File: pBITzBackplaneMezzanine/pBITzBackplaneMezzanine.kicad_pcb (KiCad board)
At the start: 4 copper layers, 99.9 x 80.4 mm, 41 parts, among them J1 USB3_A_Stacked, J2 Conn_01x04, J3 Conn_01x04, J4 10067847-001RLF, J5 Conn_02x10_Odd_Even, U1 FE1.1S-BSOP28BCN, U2 MAX3421EETJ_T, U3 CD74HC4050M96, U4 CD74HC4050M96, Y1 ABL-12.000MHZ-B2, Y2 ABL-12.000MHZ-B2

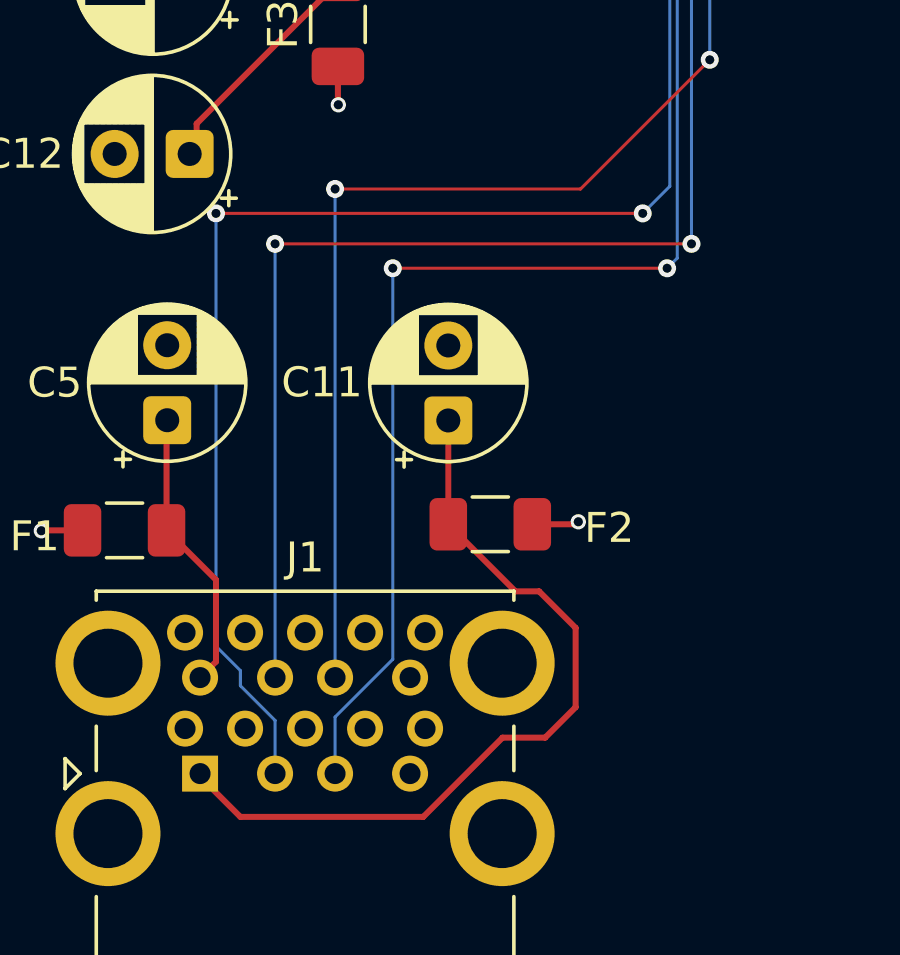
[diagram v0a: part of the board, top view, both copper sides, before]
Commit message: First pass of validation
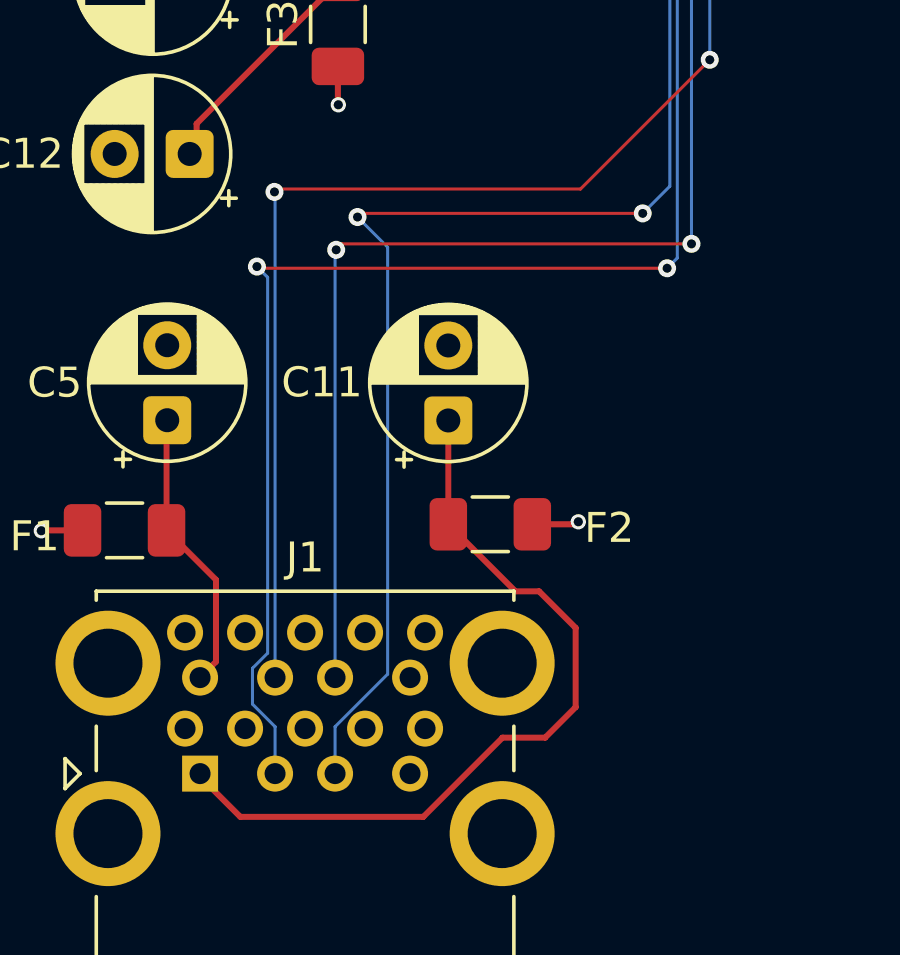
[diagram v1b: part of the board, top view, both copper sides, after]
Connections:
- J1 pad 11: /USBPorts/DP2 -> /USBPorts/DM2
- J1 pad 12: /USBPorts/DM2 -> /USBPorts/DP2
- J1 pad 2: /USBPorts/DP1 -> /USBPorts/DM1
- J1 pad 3: /USBPorts/DM1 -> /USBPorts/DP1
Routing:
- net /USBPorts/DM1: track 59.1 -> 63.6 mm
- net /USBPorts/DP1: track 63.3 -> 58.8 mm
- net /USBPorts/DP2: track 61.0 -> 58.9 mm
- net /USBPorts/DM2: track 58.7 -> 60.7 mm
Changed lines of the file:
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@@
 			(layers "*.Cu" "*.Mask")
 			(remove_unused_layers no)
-			(net "/USBPorts/DP1")
+			(net "/USBPorts/DM1")
 			(pinfunction "D1-_2")
 			(pintype "bidirectional")
@@
 			(layers "*.Cu" "*.Mask")
 			(remove_unused_layers no)
-			(net "/USBPorts/DM1")
+			(net "/USBPorts/DP1")
 			(pinfunction "D1+_3")
 			(pintype "bidirectional")
@@
 			(layers "*.Cu" "*.Mask")
 			(remove_unused_layers no)
-			(net "/USBPorts/DP2")
+			(net "/USBPorts/DM2")
 			(pinfunction "D2-_11")
 			(pintype "bidirectional")
@@
 			(layers "*.Cu" "*.Mask")
 			(remove_unused_layers no)
-			(net "/USBPorts/DM2")
+			(net "/USBPorts/DP2")
 			(pinfunction "D2+_12")
 			(pintype "bidirectional")
@@
 			)
 		)
-		(property "KiLib_Generator" "mounting_hardware/mounting_hole"
-			(at 0 0 0)
-			(layer "F.SilkS")
-			(hide yes)
-			(effects
-				(font
-					(size 1 1)
-					(thickness 0.15)
-				)
-			)
-		)
 		(property ki_fp_filters "MountingHole*Pad*")
 		(sheetname "/MezzanineConnector/")
@@
 			)
 		)
-		(property "KiLib_Generator" "connector/pin_header_socket"
-			(at 0 0 90)
-			(layer "F.SilkS")
-			(hide yes)
-			(effects
-				(font
-					(size 1 1)
-					(thickness 0.15)
-				)
-			)
-		)
 		(property "Field5" ""
 			(at 0 0 90)
@@
 			)
 		)
-		(property "KiLib_Generator" "mounting_hardware/mounting_hole"
-			(at 0 0 0)
-			(layer "F.SilkS")
-			(hide yes)
-			(effects
-				(font
-					(size 1 1)
-					(thickness 0.15)
-				)
-			)
-		)
 		(property ki_fp_filters "MountingHole*Pad*")
 		(sheetname "/MezzanineConnector/")
@@
 			)
 		)
-		(property "KiLib_Generator" "mounting_hardware/mounting_hole"
-			(at 0 0 0)
-			(layer "F.SilkS")
-			(hide yes)
-			(effects
-				(font
-					(size 1 1)
-					(thickness 0.15)
-				)
-			)
-		)
 		(property ki_fp_filters "MountingHole*Pad*")
 		(sheetname "/MezzanineConnector/")
@@
 			)
 		)
-		(property "KiLib_Generator" "mounting_hardware/mounting_hole"
-			(at 0 0 0)
-			(layer "F.SilkS")
-			(hide yes)
-			(effects
-				(font
-					(size 1 1)
-					(thickness 0.15)
-				)
-			)
-		)
 		(property ki_fp_filters "MountingHole*Pad*")
 		(sheetname "/MezzanineConnector/")
@@
 	)
 	(segment
-		(start 423.3092 187.4824)
+		(start 428.148799 187.4824)
 		(end 437.5332 187.4824)
 		(width 0.1016)
@@
 		(net "/USBPorts/DP1")
 	)
+	(segment
+		(start 428.0266 187.604599)
+		(end 428.148799 187.4824)
+		(width 0.1016)
+		(layer "F.Cu")
+		(net "/USBPorts/DP1")
+	)
 	(via
 		(at 433.6106 165.962199)
@@
 	)
 	(via
-		(at 423.3092 187.4824)
+		(at 428.0266 187.604599)
 		(size 0.6)
 		(drill 0.3)
@@
 	)
 	(segment
-		(start 424.122 203.227207)
-		(end 424.122 202.7224)
-		(width 0.1016)
-		(layer "B.Cu")
-		(net "/USBPorts/DP1")
-	)
-	(segment
 		(start 434.3864 164.562199)
 		(end 436.8364 164.562199)
@@
 	)
 	(segment
-		(start 424.122 202.7224)
-		(end 423.3092 201.9096)
+		(start 429.0308 202.839945)
+		(end 427.2784 204.592345)
 		(width 0.1016)
 		(layer "B.Cu")
@@
 	)
 	(segment
-		(start 425.2784 204.383607)
-		(end 424.122 203.227207)
+		(start 436.8364 164.562199)
+		(end 438.4364 166.162199)
 		(width 0.1016)
 		(layer "B.Cu")
@@
 	)
 	(segment
-		(start 436.8364 164.562199)
-		(end 438.4364 166.162199)
+		(start 438.4364 186.5792)
+		(end 437.5332 187.4824)
 		(width 0.1016)
 		(layer "B.Cu")
@@
 	)
 	(segment
-		(start 438.4364 186.5792)
-		(end 437.5332 187.4824)
+		(start 427.2784 204.592345)
+		(end 427.2784 206.1564)
 		(width 0.1016)
 		(layer "B.Cu")
@@
 	)
 	(segment
-		(start 433.6364 165.312199)
-		(end 434.3864 164.562199)
+		(start 428.0266 187.604599)
+		(end 429.0308 188.608799)
 		(width 0.1016)
 		(layer "B.Cu")
@@
 	)
 	(segment
-		(start 425.2784 206.1564)
-		(end 425.2784 204.383607)
+		(start 433.6364 165.312199)
+		(end 434.3864 164.562199)
 		(width 0.1016)
 		(layer "B.Cu")
@@
 	)
 	(segment
-		(start 423.3092 201.9096)
-		(end 423.3092 187.4824)
+		(start 429.0308 188.608799)
+		(end 429.0308 202.839945)
 		(width 0.1016)
 		(layer "B.Cu")
@@
 	)
 	(segment
-		(start 429.202 189.3112)
+		(start 424.6738 189.255599)
+		(end 424.729401 189.3112)
+		(width 0.1016)
+		(layer "F.Cu")
+		(net "/USBPorts/DM1")
+	)
+	(segment
+		(start 424.729401 189.3112)
 		(end 438.346 189.3112)
 		(width 0.1016)
@@
 	)
 	(via
-		(at 429.202 189.3112)
+		(at 424.6738 189.255599)
 		(size 0.6)
 		(drill 0.3)
@@
 	)
 	(segment
-		(start 429.202 189.3112)
-		(end 429.202 202.346599)
+		(start 425.0308 189.612599)
+		(end 425.0308 202.139945)
 		(width 0.1016)
 		(layer "B.Cu")
@@
 	)
 	(segment
+		(start 425.2784 204.592345)
+		(end 425.2784 206.1564)
+		(width 0.1016)
+		(layer "B.Cu")
+		(net "/USBPorts/DM1")
+	)
+	(segment
 		(start 433.7896 164.358999)
 		(end 436.920568 164.358999)
@@
 	)
 	(segment
-		(start 427.2784 204.270199)
-		(end 427.2784 206.1564)
+		(start 425.0308 202.139945)
+		(end 424.526 202.644745)
 		(width 0.1016)
 		(layer "B.Cu")
@@
 	)
 	(segment
+		(start 424.526 202.644745)
+		(end 424.526 203.839945)
+		(width 0.1016)
+		(layer "B.Cu")
+		(net "/USBPorts/DM1")
+	)
+	(segment
 		(start 436.920568 164.358999)
 		(end 438.6864 166.124831)
@@
 	)
 	(segment
-		(start 438.6864 188.9708)
-		(end 438.346 189.3112)
+		(start 424.6738 189.255599)
+		(end 425.0308 189.612599)
+		(width 0.1016)
+		(layer "B.Cu")
+		(net "/USBPorts/DM1")
+	)
+	(segment
+		(start 424.526 203.839945)
+		(end 425.2784 204.592345)
 		(width 0.1016)
 		(layer "B.Cu")
@@
 	)
 	(segment
-		(start 429.202 202.346599)
-		(end 427.2784 204.270199)
+		(start 438.6864 188.9708)
+		(end 438.346 189.3112)
 		(width 0.1016)
 		(layer "B.Cu")
@@
 	)
 	(segment
-		(start 425.2784 188.4984)
+		(start 427.3154 188.696799)
+		(end 427.513799 188.4984)
+		(width 0.1016)
+		(layer "F.Cu")
+		(net "/USBPorts/DP2")
+	)
+	(segment
+		(start 427.513799 188.4984)
 		(end 439.1588 188.4984)
 		(width 0.1016)
@@
 	)
 	(via
-		(at 425.2784 188.4984)
+		(at 427.3154 188.696799)
 		(size 0.6)
 		(drill 0.3)
@@
 	)
 	(segment
-		(start 425.2784 202.9564)
-		(end 425.2784 188.4984)
+		(start 427.2784 188.733799)
+		(end 427.3154 188.696799)
 		(width 0.1016)
 		(layer "B.Cu")
@@
 	)
 	(segment
+		(start 427.2784 202.9564)
+		(end 427.2784 188.733799)
+		(width 0.1016)
+		(layer "B.Cu")
+		(net "/USBPorts/DP2")
+	)
+	(segment
 		(start 439.1588 188.4984)
 		(end 439.1588 166.309863)
@@
 	)
 	(segment
-		(start 427.2784 186.6696)
+		(start 425.258 186.766399)
+		(end 425.354799 186.6696)
+		(width 0.1016)
+		(layer "F.Cu")
+		(net "/USBPorts/DM2")
+	)
+	(segment
+		(start 425.354799 186.6696)
 		(end 435.460999 186.6696)
 		(width 0.1016)
@@
 	)
 	(via
-		(at 427.2784 186.6696)
+		(at 425.258 186.766399)
 		(size 0.6)
 		(drill 0.3)
@@
 	)
 	(segment
-		(start 427.2784 186.6696)
-		(end 427.2784 202.9564)
-		(width 0.1016)
-		(layer "B.Cu")
-		(net "/USBPorts/DM2")
-	)
-	(segment
 		(start 437.1364 163.912199)
 		(end 432.3364 163.912199)
@@
 		(width 0.1016)
 		(layer "B.Cu")
+		(net "/USBPorts/DM2")
+	)
+	(segment
+		(start 425.2784 186.786799)
+		(end 425.2784 202.9564)
+		(width 0.1016)
+		(layer "B.Cu")
+		(net "/USBPorts/DM2")
+	)
+	(segment
+		(start 425.258 186.766399)
+		(end 425.2784 186.786799)
+		(width 0.1016)
+		(layer "B.Cu")
